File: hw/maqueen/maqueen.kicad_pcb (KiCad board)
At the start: 2 copper layers, 80 x 75 mm, 29 parts, among them IC1 MSP430FR2355TPT, J1 conn_DFrobot, J2 ESP01, J3 SBW, SW1 RST, U1 LMV324, Y1 Crystal

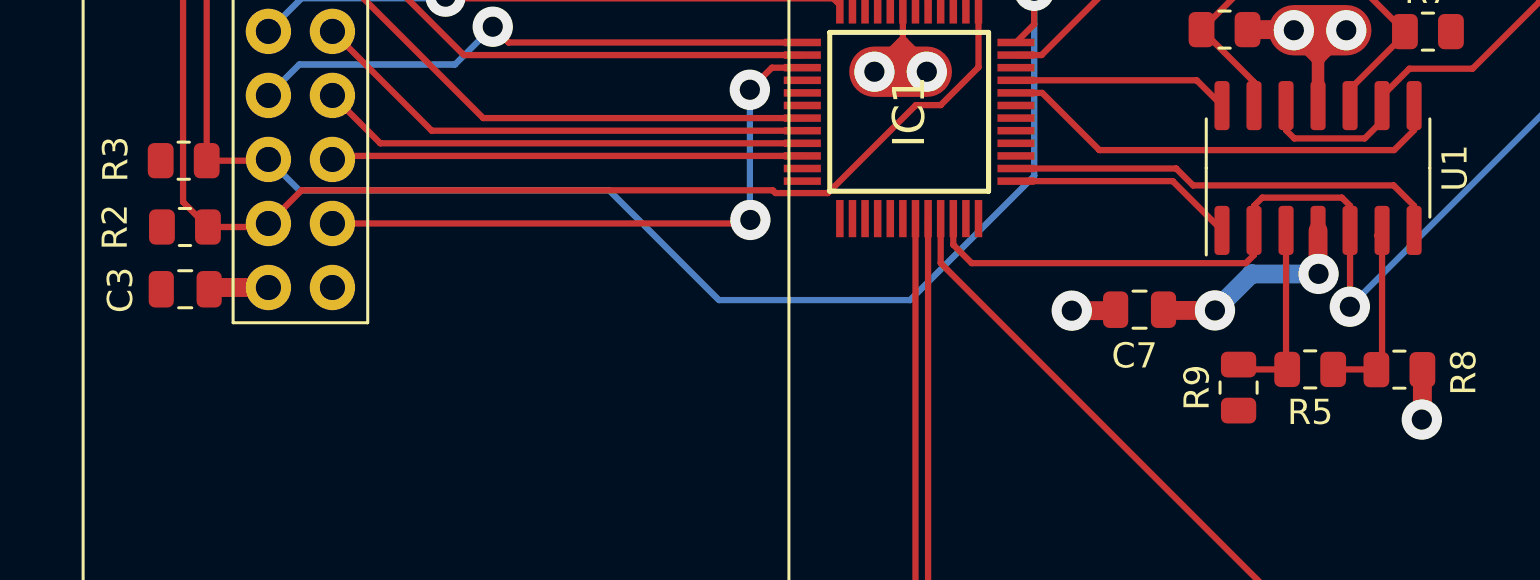
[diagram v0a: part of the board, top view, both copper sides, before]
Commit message: testing points & minor adjustements
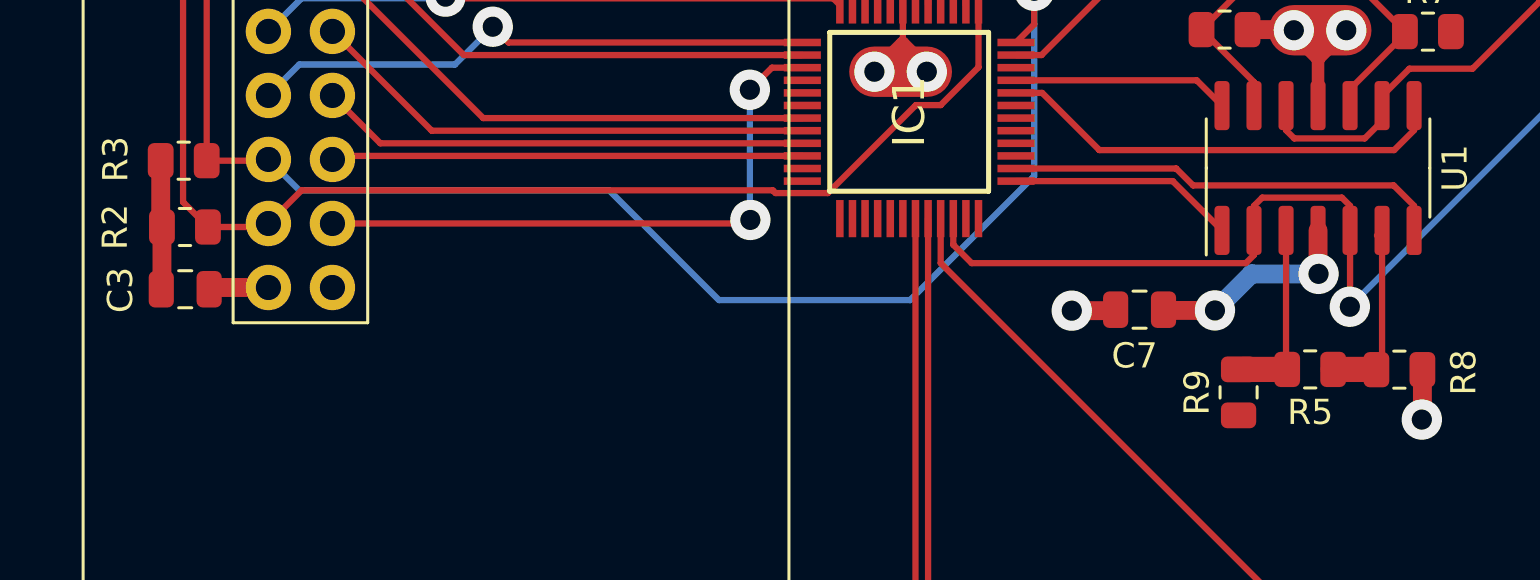
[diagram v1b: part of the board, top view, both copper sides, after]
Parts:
- moved R9 0.19 mm to (163.0, 111.7)
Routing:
- net +3.3V: track 36.3 -> 41.4 mm
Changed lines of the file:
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@@
   )
   (footprint "Resistor_SMD:R_0805_2012Metric" (layer "F.Cu")
-    (at 163.0275 111.51 90)
+    (at 163.0275 111.7 90)
     (descr "Resistor SMD 0805 (2012 Metric), square (rectangular) end terminal, IPC_7351 nominal, (Body size source: IPC-SM-782 page 72, https://www.pcb-3d.com/wordpress/wp-content/uploads/ipc-sm-782a_amendment_1_and_2.pdf), generated with kicad-footprint-generator")
     (tags "resistor")
@@
   (segment (start 144.5495 103.685) (end 144.6595 103.795) (width 0.25) (layer "F.Cu") (net 1))
   (segment (start 144.6595 103.795) (end 146.735 103.795) (width 0.25) (layer "F.Cu") (net 1))
+  (segment (start 120.3175 107.5825) (end 120.29 107.61) (width 0.75) (layer "F.Cu") (net 2))
   (segment (start 162.09 108.45) (end 160.08 108.45) (width 0.75) (layer "F.Cu") (net 2))
   (segment (start 160.11 108.45) (end 160.07 108.49) (width 0.75) (layer "F.Cu") (net 2))
+  (segment (start 120.3175 105.14) (end 120.3175 107.5825) (width 0.75) (layer "F.Cu") (net 2))
   (segment (start 160.08 108.45) (end 160.05 108.42) (width 0.75) (layer "F.Cu") (net 2))
   (segment (start 166.18 106.98) (end 166.2 107) (width 0.75) (layer "F.Cu") (net 2))
@@
   (segment (start 151.12 89.96) (end 151.07 89.91) (width 0.75) (layer "F.Cu") (net 2))
   (segment (start 151.114504 92.774504) (end 150.21 93.679008) (width 0.25) (layer "F.Cu") (net 2))
+  (segment (start 120.2675 105.09) (end 120.3175 105.14) (width 0.75) (layer "F.Cu") (net 2))
   (segment (start 150.21 93.679008) (end 150.21 96.332) (width 0.25) (layer "F.Cu") (net 2))
   (segment (start 127.055 70.83) (end 127.38 71.155) (width 0.75) (layer "F.Cu") (net 2))
+  (segment (start 120.2675 102.51) (end 120.2675 105.09) (width 0.75) (layer "F.Cu") (net 2))
   (segment (start 124.47 70.83) (end 127.055 70.83) (width 0.75) (layer "F.Cu") (net 2))
   (via (at 137.28 82.22) (size 1.6) (drill 0.8) (layers "F.Cu" "B.Cu") (free) (net 2))
@@
   (segment (start 160.415 103.32) (end 154.198 103.32) (width 0.25) (layer "F.Cu") (net 25))
   (segment (start 164.91 110.745) (end 164.955 110.79) (width 0.25) (layer "F.Cu") (net 33))
-  (segment (start 164.955 110.79) (end 163.22 110.79) (width 0.25) (layer "F.Cu") (net 33))
+  (segment (start 164.955 110.79) (end 163.22 110.79) (width 1) (layer "F.Cu") (net 33))
   (segment (start 164.9775 105.3425) (end 164.91 105.275) (width 0.25) (layer "F.Cu") (net 33))
   (segment (start 163.22 110.79) (end 163.0275 110.5975) (width 0.25) (layer "F.Cu") (net 33))
@@
   (segment (start 168.485 110.79) (end 168.495 110.8) (width 0.25) (layer "F.Cu") (net 34))
   (segment (start 168.5175 105.4775) (end 168.72 105.275) (width 0.25) (layer "F.Cu") (net 34))
-  (segment (start 166.78 110.79) (end 168.485 110.79) (width 0.25) (layer "F.Cu") (net 34))
+  (segment (start 166.78 110.79) (end 168.485 110.79) (width 1) (layer "F.Cu") (net 34))
   (segment (start 169.6275 97.4925) (end 169.6275 97.39) (width 0.25) (layer "F.Cu") (net 35))
   (segment (start 167.45 99.67) (end 169.6275 97.4925) (width 0.25) (layer "F.Cu") (net 35))
